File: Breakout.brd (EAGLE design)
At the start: 80 x 100 mm, 177 parts, among them IC1 LM337LZ, IC2 78L05SMD, U1 ADS131E08, U11 TC1014, U12 LTC6655, U2 TLV433, U3 TLV433, U4 TLV433, U5 TLV433, U6 TLV433, U7 TLV433, U8 TLV433, U9 TLV433, X1 X-MHz, X3 BU-SMA-V

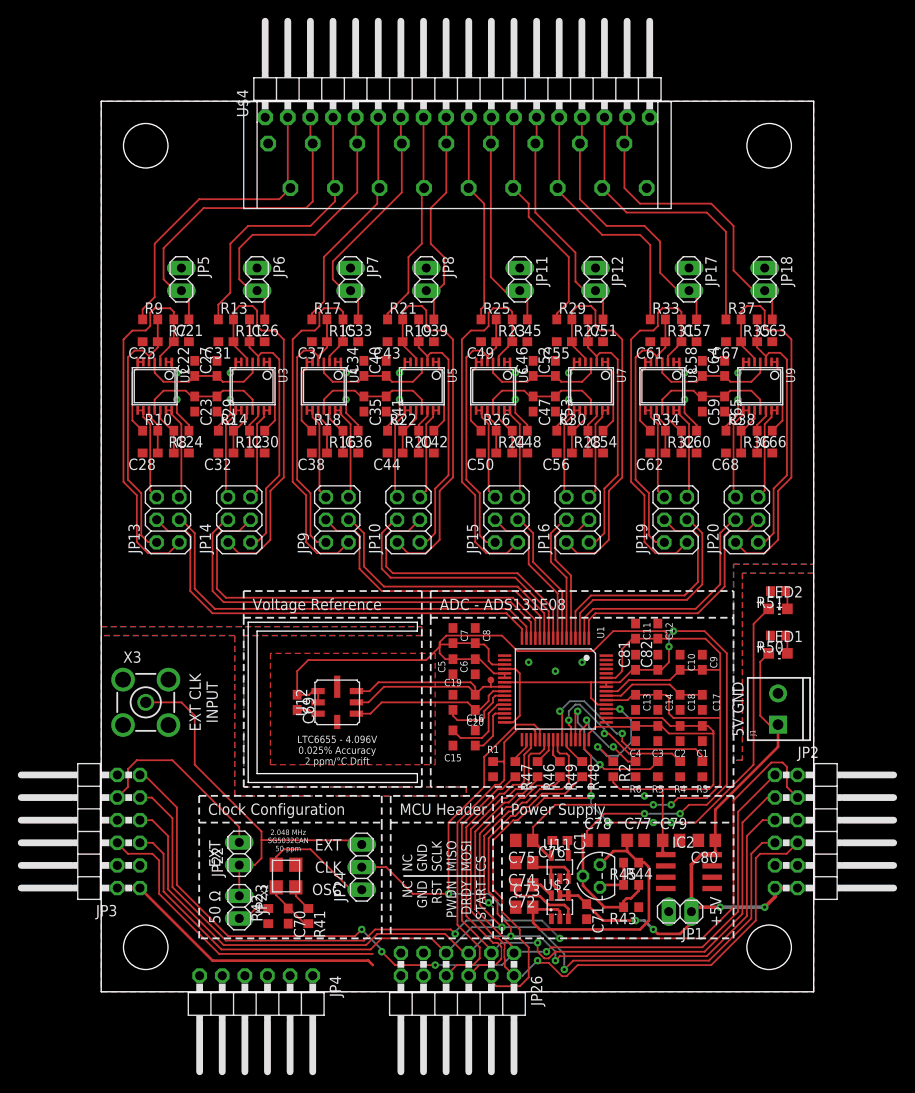
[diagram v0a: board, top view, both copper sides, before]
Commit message: Op-amp Power Routed
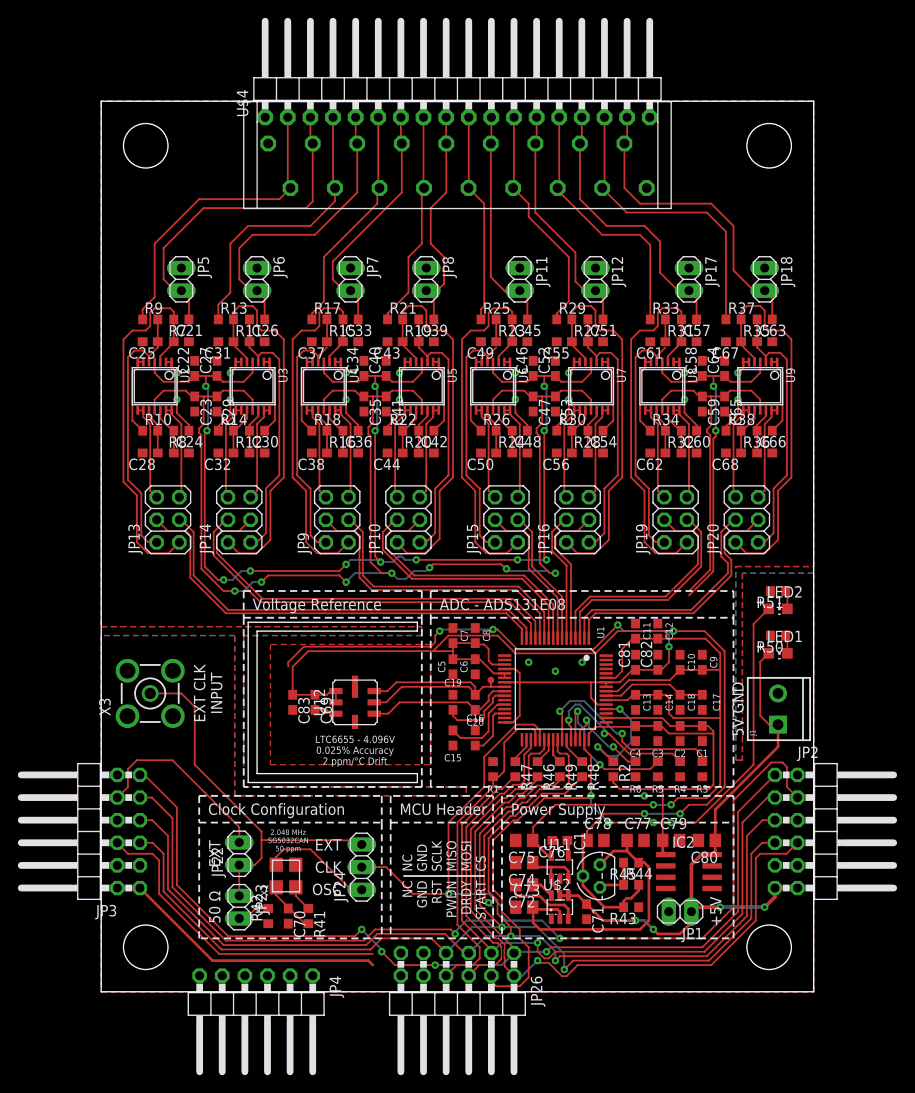
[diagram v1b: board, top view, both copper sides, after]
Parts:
- added C83: 1µ, resistor:C0603
- moved C69 2.00 mm to (24.0, 32.5)
- moved U12 2.00 mm to (28.5, 32.5)
- moved X3 1.12 mm to (5.50, 33.5), turned to 90 degrees
- turned R1 to 90 degrees
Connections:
- new net PAS3: C37.1, JP9.2, R17.2, U4.5
- new net PAS4: C43.1, JP10.2, R21.2, U5.5
- new net PAS5: C49.1, JP15.2, R25.2, U6.5
- new net PAS6: C55.1, JP16.2, R29.2, U7.5
- new net PAS7: C61.1, JP19.2, R33.2, U8.5
- new net PAS8: C67.1, JP20.2, R37.2, U9.5
- net PAS1: no longer C37.1, C49.1, C61.1, JP15.2, JP19.2, JP9.2, R17.2, R25.2, R33.2, U4.5, U6.5, U8.5
- net PAS2: no longer C43.1, C55.1, C67.1, JP10.2, JP16.2, JP20.2, R21.2, R29.2, R37.2, U5.5, U7.5, U9.5
- net VCC: now also C83.1
- net VSS: now also C83.2
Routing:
- net VSS: track 171.7 -> 346.9 mm, vias 4 -> 14
- net VCC: track 218.9 -> 352.5 mm, vias 2 -> 17
- net PAS2: track 175.1 -> 43.8 mm
- net PAS1: track 123.2 -> 30.8 mm
- net PAS6: track 0.00 -> 42.9 mm
- net PAS8: track 0.00 -> 42.9 mm
- net PAS4: track 0.00 -> 42.9 mm
- net PAS3: track 0.00 -> 30.2 mm
- net PAS7: track 0.00 -> 30.2 mm
- net PAS5: track 0.00 -> 30.2 mm
- net VREF: track 34.1 -> 30.1 mm
- net AIN2: track 47.9 -> 45.3 mm
- net -AIN2: track 49.7 -> 47.3 mm
- net -AIN7: track 26.0 -> 24.7 mm
- net RST: track 38.8 -> 37.6 mm
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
